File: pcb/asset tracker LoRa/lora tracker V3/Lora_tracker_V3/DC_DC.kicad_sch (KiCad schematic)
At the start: 11 parts, among them J1 Screw_Terminal_01x02, U1 MAX5035AUSA

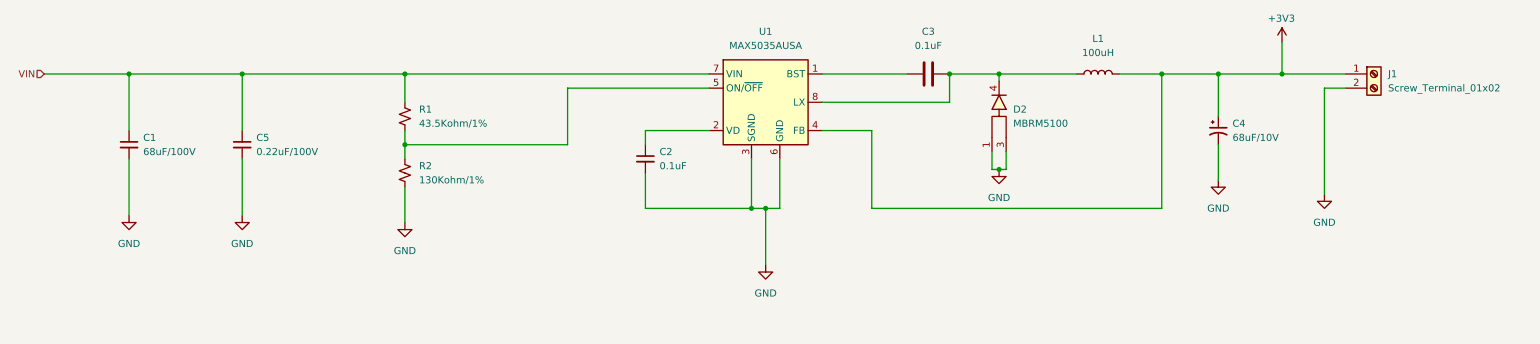
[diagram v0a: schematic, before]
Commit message: eadf
sdfv
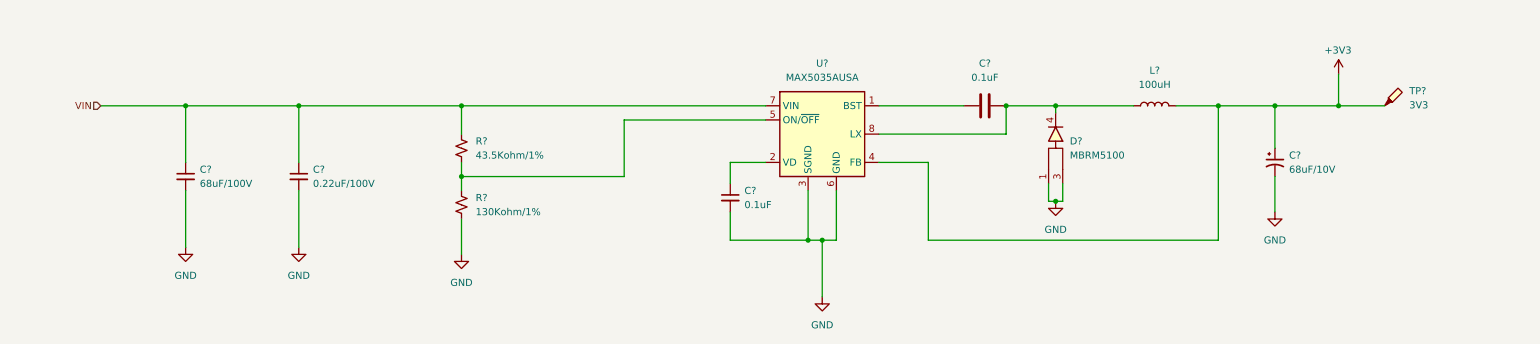
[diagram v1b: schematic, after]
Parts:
- removed C1: 68uF/100V, vanalles:CAPAE1030X1050D1200L350X90N, symbol Device:C_Small
- removed C2: 0.1uF, vanalles:0603, symbol Device:C_Small
- removed C3: 0.1uF, vanalles:0603, symbol Device:C
- removed C4: 68uF/10V, vanalles:CAPAE1030X1050D1200L350X90N, symbol Device:C_Polarized_Small_US
- removed C5: 0.22uF/100V, vanalles:CAPAE1030X1050D1200L350X90N, symbol Device:C_Small
- removed D2: MBRM5100, halfgeleiders:DPAK, symbol Halfgelijders:diode4
- removed J1: Screw_Terminal_01x02, connectors_user:2pin_screw_vast, symbol Connector:Screw_Terminal_01x02
- removed L1: 100uH, vanalles:DO5022p, symbol Device:L
- removed R1: 43.5Kohm/1%, vanalles:0603, symbol Device:R_Small_US
- removed R2: 130Kohm/1%, vanalles:0603, symbol Device:R_Small_US
- removed U1: MAX5035AUSA, halfgeleiders:soic HV clearance, symbol Regulator_Switching:MAX5035AUSA
- added C?: 68uF/10V, vanalles:CAPAE1030X1050D1200L350X90N, symbol Device:C_Polarized_Small_US
- added C?: 0.22uF/100V, vanalles:CAPAE1030X1050D1200L350X90N, symbol Device:C_Small
- added C?: 0.1uF, vanalles:0603, symbol Device:C
- added C?: 68uF/100V, vanalles:CAPAE1030X1050D1200L350X90N, symbol Device:C_Small
- added C?: 0.1uF, vanalles:0603, symbol Device:C_Small
- added D?: MBRM5100, halfgeleiders:DPAK, symbol Halfgelijders:diode4
- added L?: 100uH, vanalles:DO5022p, symbol Device:L
- added R?: 130Kohm/1%, vanalles:0603, symbol Device:R_Small_US
- added R?: 43.5Kohm/1%, vanalles:0603, symbol Device:R_Small_US
- added TP?: 3V3, symbol Connector:Test_Point_Probe
- added U?: MAX5035AUSA, halfgeleiders:soic HV clearance, symbol Regulator_Switching:MAX5035AUSA
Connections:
- net +3V3: now also C?.1, L?.2, TP?.1, U?.4 (FB)
- net GND: now also C?.2, C?.2, C?.2, C?.2, D?.1, D?.3, R?.2, U?.3 (SGND), U?.6 (GND)
- net VIN: now also C?.1, C?.1, R?.1, U?.7 (VIN)
- new net: C?.1, U?.1 (BST)
- new net: C?.2, D?.4, L?.1, U?.8 (LX)
- new net: R?.1, R?.2, U?.5 (ON/~{OFF})
- new net: C?.1, U?.2 (VD)
